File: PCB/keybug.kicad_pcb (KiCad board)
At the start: 2 copper layers, 21 x 96.5 mm, 8 parts, among them U2 rp2040-zero

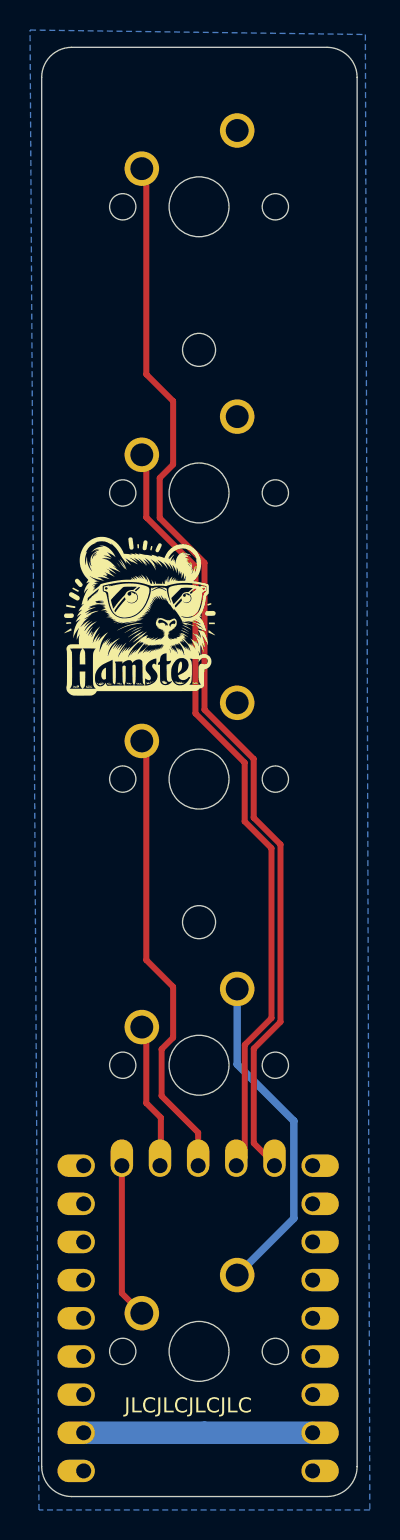
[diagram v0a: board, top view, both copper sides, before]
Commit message: Add LEDs to PCB
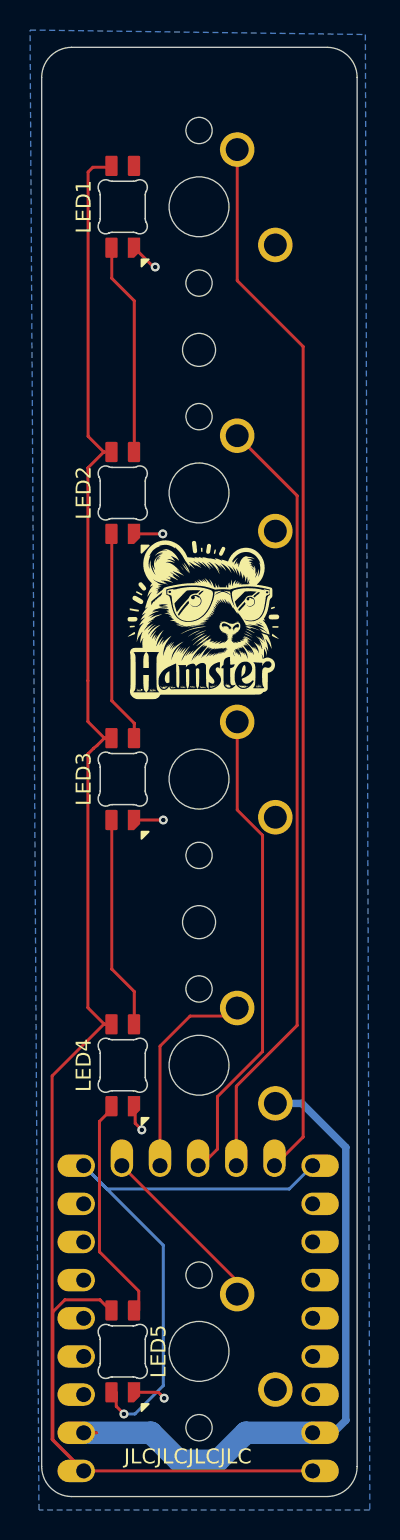
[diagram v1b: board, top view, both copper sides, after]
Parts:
- added LED1: MX_SK6812MINI-E, PCM_marbastlib-mx:LED_MX_6028R-ROT, F.Cu at (91.9, 43.6)
- added LED2: MX_SK6812MINI-E, PCM_marbastlib-mx:LED_MX_6028R-ROT, F.Cu at (91.9, 62.7)
- added LED3: MX_SK6812MINI-E, PCM_marbastlib-mx:LED_MX_6028R-ROT, F.Cu at (91.9, 81.7)
- added LED4: MX_SK6812MINI-E, PCM_marbastlib-mx:LED_MX_6028R-ROT, F.Cu at (91.9, 100.8)
- added LED5: MX_SK6812MINI-E, PCM_marbastlib-mx:LED_MX_6028R-ROT, F.Cu at (91.9, 119.8)
- turned MX1 to -90 degrees
- turned MX2 to -90 degrees
- turned MX3 to -90 degrees
- turned MX4 to -90 degrees
- turned MX5 to -90 degrees
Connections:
- U2 pad 1: unconnected-(U2-0-Pad1) -> VDD
- U2 pad 15: unconnected-(U2-14-Pad15) -> RGB
- U2 pad 23: unconnected-(U2-5V-Pad23) -> VDD
- U2 pad 9: unconnected-(U2-8-Pad9) -> RGB
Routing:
- net VDD: track 0.00 -> 126.5 mm
- net RGB: track 0.00 -> 38.4 mm, vias 0 -> 1
- net GND: track 38.0 -> 54.8 mm, vias 0 -> 5
- net Net-(LED4-DIN): track 0.00 -> 14.9 mm
- net Net-(LED1-DIN): track 0.00 -> 14.5 mm
- net Net-(LED2-DIN): track 0.00 -> 14.2 mm
- net Net-(LED3-DIN): track 0.00 -> 14.2 mm
- net SW4: track 9.69 -> 14.1 mm
- net SW1: track 72.2 -> 70.3 mm
- net SW5: track 10.4 -> 11.7 mm
